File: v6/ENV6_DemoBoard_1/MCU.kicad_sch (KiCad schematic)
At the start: 50 parts, among them J101 Conn_01x03_Pin, J102 Conn_01x20_Pin, J103 Conn_01x20_Pin, U101 RP235xB, U102 W25Q16JVUXIQ, U103 Pi-Radio, Y101 KX7_QRZ

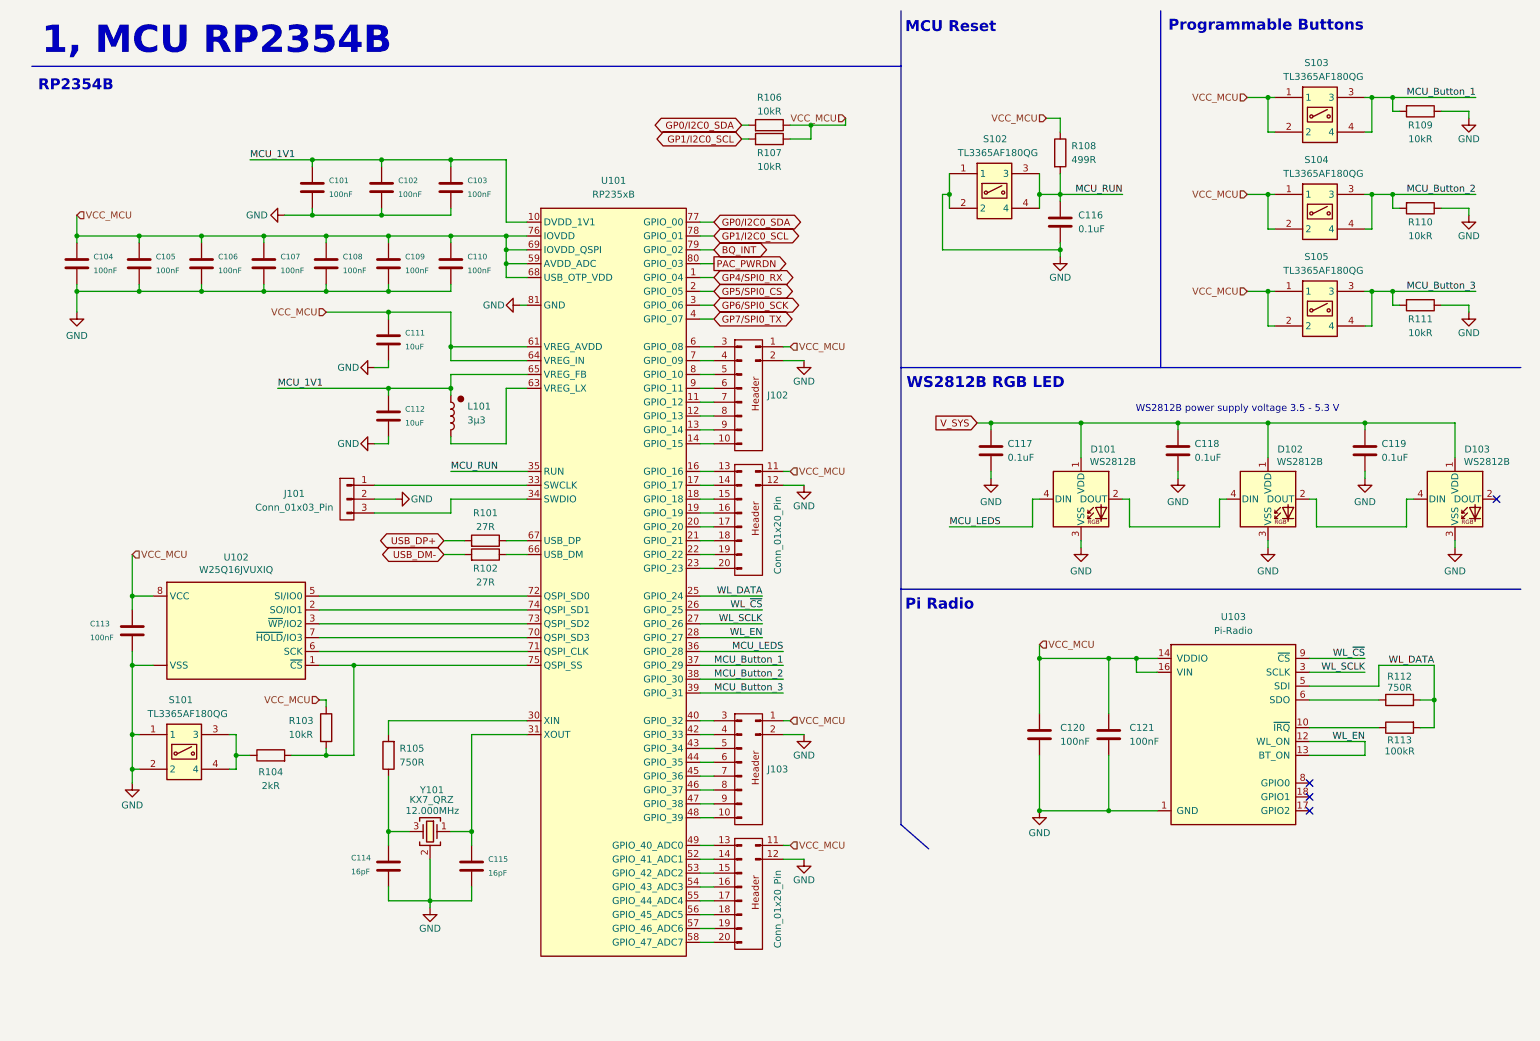
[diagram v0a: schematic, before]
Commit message: ENV6 (test): Changes after first review
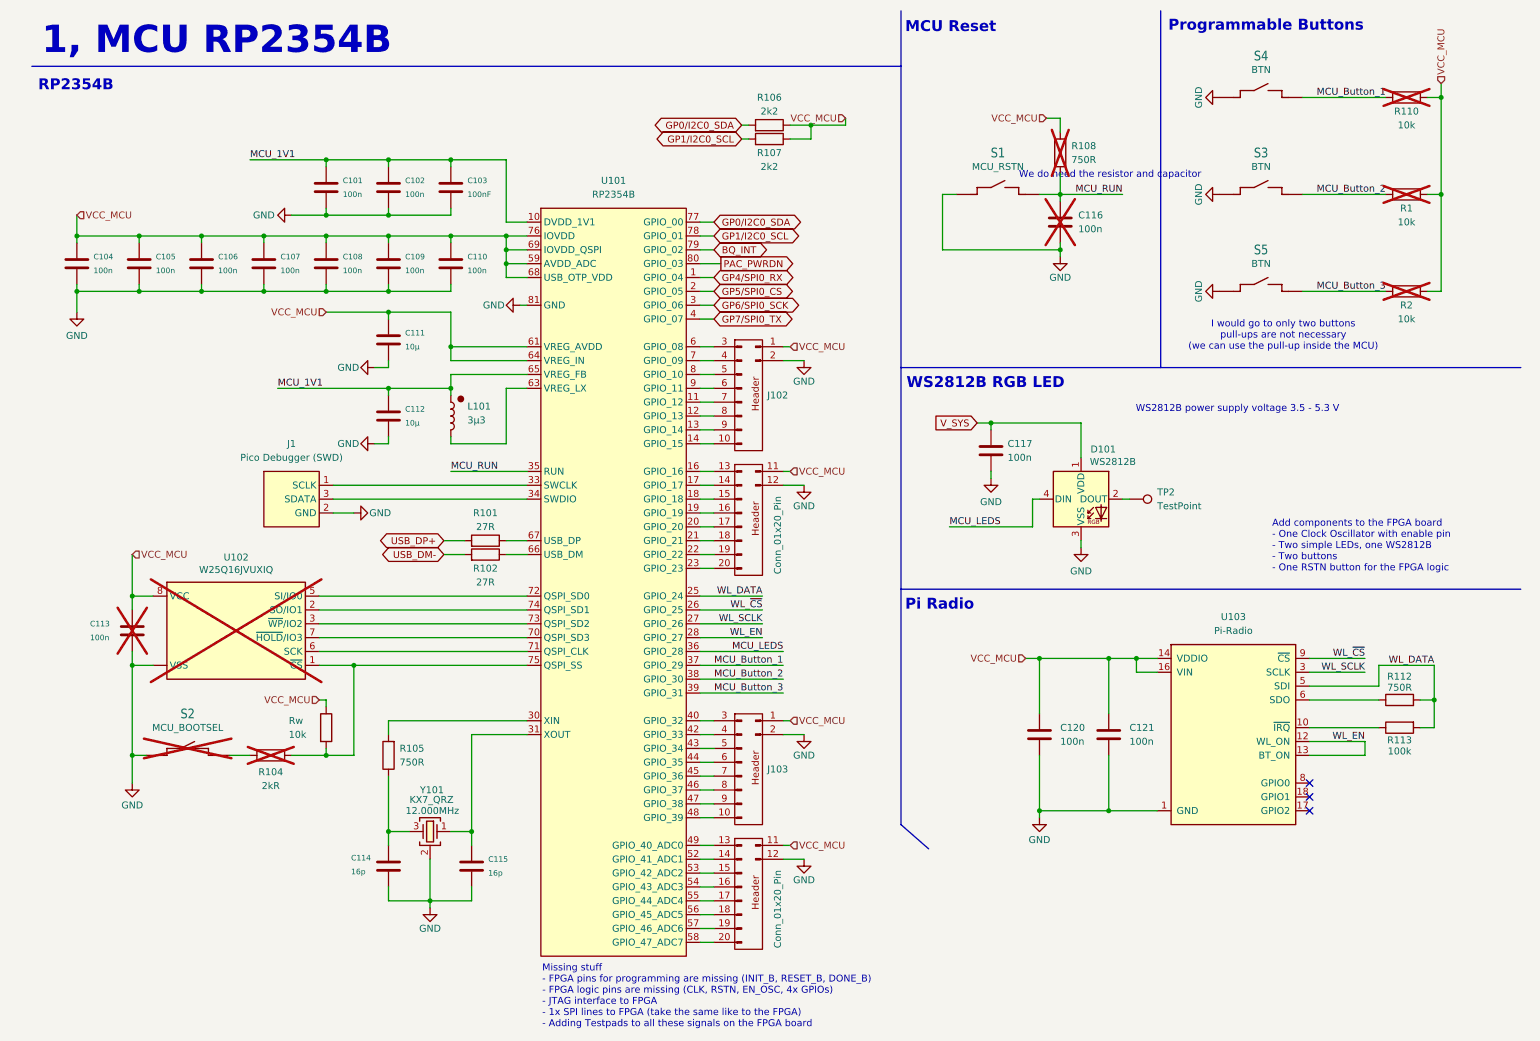
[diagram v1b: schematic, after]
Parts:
- removed C118, C119: 0.1uF, Capacitor_SMD:C_0402_1005Metric, symbol passive:C0402
- removed D102, D103: WS2812B, LED_SMD:LED_WS2812B_PLCC4_5.0x5.0mm_P3.2mm, symbol LED:WS2812B
- removed J101: Conn_01x03_Pin, Connector_PinSocket_2.54mm:PinSocket_1x03_P2.54mm_Vertical, symbol Connector:Conn_01x03_Pin
- removed R109, R111: 10kR, Resistor_SMD:R_0402_1005Metric, symbol Device:R
- removed S101, S102, S103, S104, S105: TL3365AF180QG, ui_stuff:TL3365AF180QG, symbol TL3365AF180QG:TL3365AF180QG
- added J1: Pico Debugger (SWD), Connector_PinHeader_2.54mm:PinHeader_1x03_P2.54mm_Vertical, symbol mcu_rpi_pico:PicoDebuggerSWD
- added R1, R2: 10k, Resistor_SMD:R_0402_1005Metric, symbol Device:R
- added S1: MCU_RSTN, connectors:TACTILE-SWITCH, symbol connectors:Tactile Button
- added S2: MCU_BOOTSEL, connectors:TACTILE-SWITCH, symbol connectors:Tactile Button
- added S3, S4, S5: BTN, connectors:TACTILE-SWITCH, symbol connectors:Tactile Button
- added TP2: TestPoint, custom_library:TestPoint_Pad_D1.0mm, symbol passive:TestPoint
- C101, C102, C104, C105, C106, C107, C108, C109, C110, C120, C121: value 100nF -> 100n
- C111, C112: value 10uF -> 10µ
- C113: value 100nF -> 100n; now not fitted; now left out of the parts list
- C114, C115: value 16pF -> 16p
- C116: value 0.1uF -> 100n; now not fitted; now left out of the parts list
- C117: value 0.1uF -> 100n
- R104, U102: now not fitted; now left out of the parts list
- R106, R107: value 10kR -> 2k2
- R108: value 499R -> 750R; now not fitted; now left out of the parts list
- R110: value 10kR -> 10k; now not fitted; now left out of the parts list
- R113: value 100kR -> 100k
- Rw: renamed from R103; value 10kR -> 10k
- U101: value RP235xB -> RP2354B
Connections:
- net GND: now also J1.2 (GND), S1.1, S1.2 (1), S2.1, S2.2 (1), S3.1, S3.2 (1), S4.1, S4.2 (1), S5.1, S5.2 (1); no longer R110.1
- net IOVDD: now also R110.1, R1.1, R2.1
- net MCU_Button_1: now also R110.2, S4.3 (2), S4.4 (2)
- net MCU_Button_2: now also R1.2, S3.3 (2), S3.4 (2); no longer R110.2
- net MCU_Button_3: now also R2.2, S5.3 (2), S5.4 (2)
- net MCU_RUN: now also S1.3 (2), S1.4 (2)
- net at R104.1: now also S2.3 (2), S2.4 (2)
- net at U101.33 (SWCLK): now also J1.1 (SCLK)
- net at U101.34 (SWDIO): now also J1.3 (SDATA)
- net at D101.2 (DOUT): now also TP2.1
- no-connect marks 4 -> 3
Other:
- note added: "Add components to the FPGA board - One Clock Oscillator with enable pin - Two simple LEDs, one WS2812B - Two buttons - One RSTN button for the FPGA logic"
- note added: "I would go to only two buttons pull-ups are not necessary (we can use the pull-up inside the MCU)"
- note added: "Missing stuff - FPGA pins for programming are missing (INIT_B, RESET_B, DONE_B) - FPGA logic pins are missing (CLK, RSTN, EN_OSC, 4x GPIOs) - JTAG interface to FPGA - 1x SPI lines to FPGA (take the same like to the FPGA) - Adding Testpads to all these signals on the FPGA board"
- note added: "We do need the resistor and capacitor"
- moved on the sheet: C101, C102
